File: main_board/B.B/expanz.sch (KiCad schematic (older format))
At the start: 22 parts, among them J1 Conn_01x04, J4 Conn_01x04, M1 Motor_DC, Q10 2N7002, Q7 SI3447CDV, U68 IRM-H936, U70 MH253ESO, U71 MH253ESO

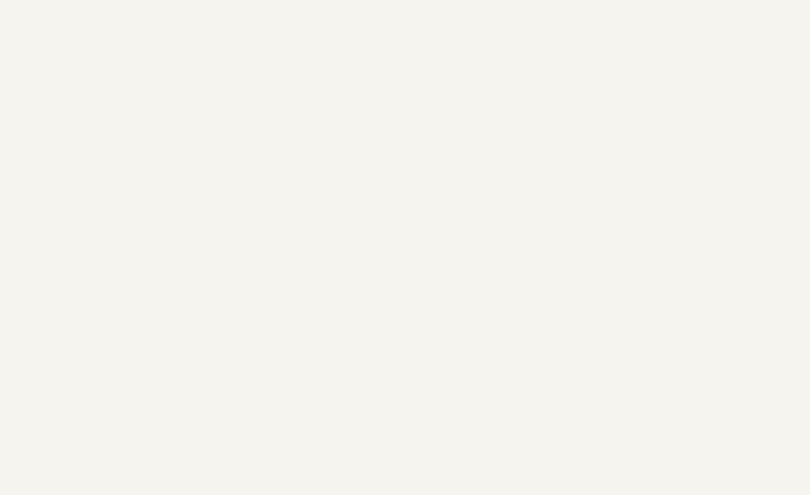
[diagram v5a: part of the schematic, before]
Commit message: opravy_a_dodatky_2
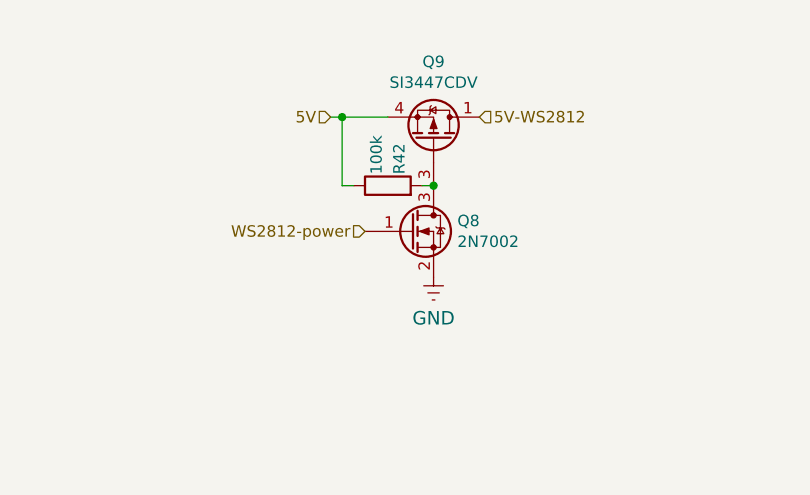
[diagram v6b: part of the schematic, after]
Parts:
- added Q8: 2N7002, Package_TO_SOT_SMD:SOT-23, symbol B.B-rescue:2N7002-Transistor_FET-B.B-rescue
- added Q9: SI3447CDV, BB:TSOP-6_1.5x3.0x0.95P, symbol B.B-rescue:Q_PMOS_DSG-B.B-rescue
- added R42: 100k, Resistor_SMD:R_0402_1005Metric, symbol B.B-rescue:R-Device-B.B-rescue
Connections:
- net 5V: now also Q9.4 (S), R42.1
- new net: Q8.3 (D), Q9.3 (G), R42.2
- new net 5V-WS2812: Q9.1 (D), Q9.2, Q9.5, Q9.6
- new net WS2812-power: Q8.1 (G)
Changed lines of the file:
@@
 EESchema Schematic File Version 4
-LIBS:B.B-cache
-EELAYER 29 0
+EELAYER 30 0
 EELAYER END
 $Descr A4 11693 8268
 encoding utf-8
-Sheet 7 8
+Sheet 8 8
 Title ""
 Date ""
@@
 $EndComp
 $Comp
+L B.B-rescue:GND-B.B-eagle-import #GND0137
+U 1 1 5F9DF814
+P 7750 3025
+AR Path="/5F9EE529/5F9DF814" Ref="#GND0137"  Part="1"
+AR Path="/5FA9DBB3/5F9DF814" Ref="#GND?"  Part="1"
+F 0 "#GND0137" H 7750 3025 50  0001 C CNN
+F 1 "GND" H 7750 2945 59  0000 C CNN
+F 2 "" H 7750 3025 50  0001 C CNN
+F 3 "" H 7750 3025 50  0001 C CNN
+	1    7750 3025
+	1    0    0    -1
+$EndComp
+Text HLabel 7950 2225 2    50   Input ~ 0
+5V-WS2812
+Text HLabel 7300 2225 0    50   Input ~ 0
+5V
+$Comp
+L B.B-rescue:R-Device-B.B-rescue R?
+U 1 1 5FAAB362
+P 7550 2525
+AR Path="/5F96CFDA/5FAAB362" Ref="R?"  Part="1"
+AR Path="/5F9EE529/5F9F24D4/5FAAB362" Ref="R?"  Part="1"
+AR Path="/5FA9DBB3/5F9F24D4/5FAAB362" Ref="R?"  Part="1"
+AR Path="/5F9EE529/5FAAB362" Ref="R42"  Part="1"
+F 0 "R42" H 7600 2475 50  0000 L CNN
+F 1 "100k" H 7600 2575 50  0000 L CNN
+F 2 "Resistor_SMD:R_0402_1005Metric" V 7480 2525 50  0001 C CNN
+F 3 "~" H 7550 2525 50  0001 C CNN
+F 4 "C25741" H 7550 2525 50  0001 C CNN "LCSC"
+	1    7550 2525
+	0    -1   -1   0
+$EndComp
+Wire Wire Line
+	7700 2525 7750 2525
+Wire Wire Line
+	7300 2225 7350 2225
+Wire Wire Line
+	7400 2525 7350 2525
+Wire Wire Line
+	7350 2525 7350 2225
+Connection ~ 7350 2225
+Wire Wire Line
+	7350 2225 7550 2225
+Text HLabel 7450 2725 0    50   Input ~ 0
+WS2812-power
+$Comp
 L B.B-rescue:MH253ESO-B.B-rescue U?
 U 1 1 5FB5B56F
@@
 $EndComp
 $Comp
+L B.B-rescue:Q_PMOS_DSG-B.B-rescue Q9
+U 1 1 602B1909
+P 7750 2325
+F 0 "Q9" V 8092 2325 50  0000 C CNN
+F 1 "SI3447CDV" V 8001 2325 50  0000 C CNN
+F 2 "BB:TSOP-6_1.5x3.0x0.95P" H 7950 2425 50  0001 C CNN
+F 3 "https://datasheet.lcsc.com/szlcsc/Vishay-Intertech-SI3447CDV-T1-E3_C145421.pdf" H 7750 2325 50  0001 C CNN
+F 4 "C144884" V 7750 2325 50  0001 C CNN "LCSC"
+	1    7750 2325
+	0    1    -1   0
+$EndComp
+$Comp
 L B.B-rescue:2N7002-Transistor_FET-B.B-rescue Q?
+U 1 1 5FBA8934
+P 7650 2725
+AR Path="/5F77B818/5FBA8934" Ref="Q?"  Part="1"
+AR Path="/5FA4C94D/5FBA8934" Ref="Q?"  Part="1"
+AR Path="/5F9EE529/5FBA8934" Ref="Q8"  Part="1"
+F 0 "Q8" H 7854 2771 50  0000 L CNN
+F 1 "2N7002" H 7854 2680 50  0000 L CNN
+F 2 "Package_TO_SOT_SMD:SOT-23" H 7850 2650 50  0001 L CIN
+F 3 "https://datasheet.lcsc.com/szlcsc/Changjiang-Electronics-Tech-CJ-CJ3134K_C110100.pdf" H 7650 2725 50  0001 L CNN
+F 4 "C8545" H 7650 2725 50  0001 C CNN "LCSC"
+F 5 "0;0;180" H 7650 2725 50  0001 C CNN "JLCPCB_CORRECTION"
+	1    7650 2725
+	1    0    0    -1
+$EndComp
+Connection ~ 7750 2525
+$Comp
+L B.B-rescue:2N7002-Transistor_FET-B.B-rescue Q?

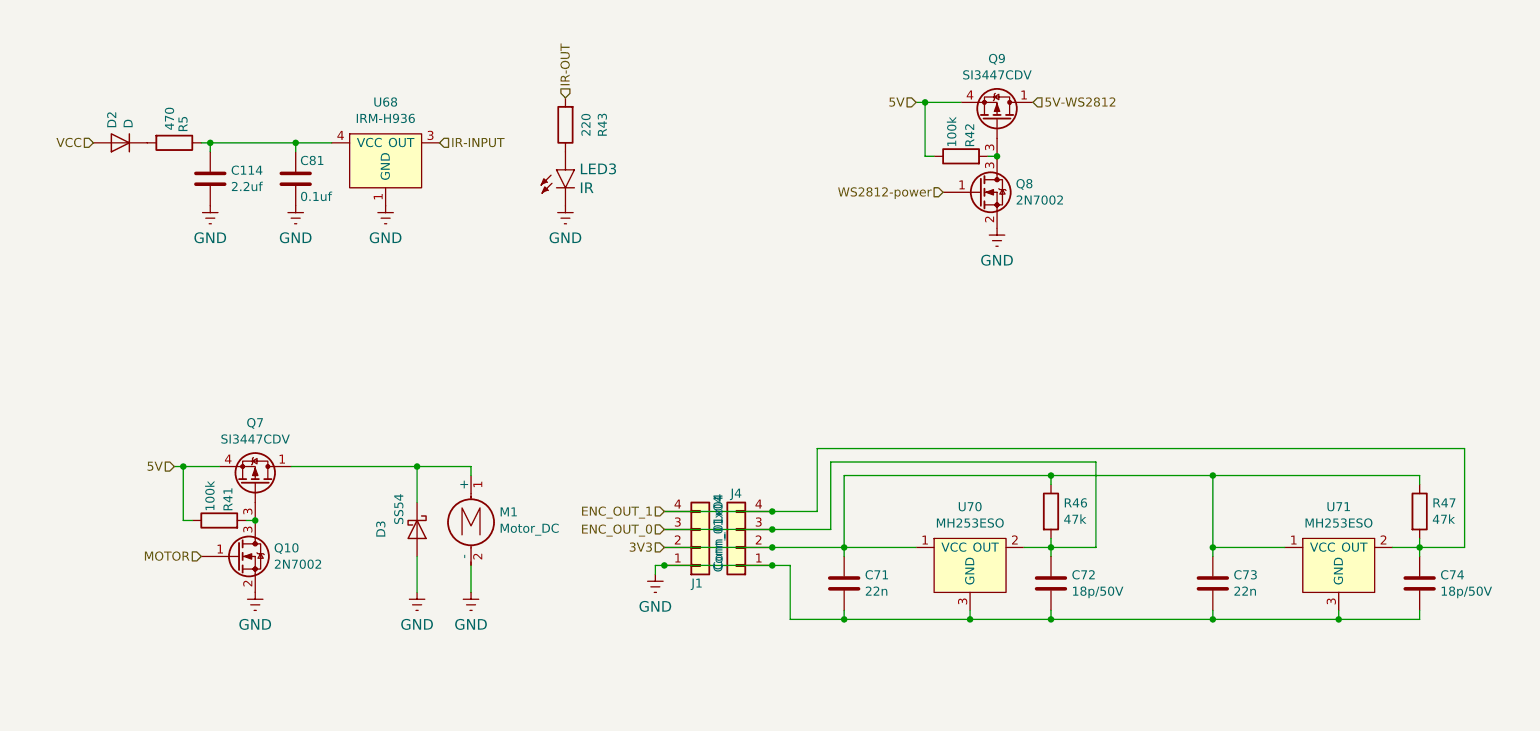
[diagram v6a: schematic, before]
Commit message: lucerna
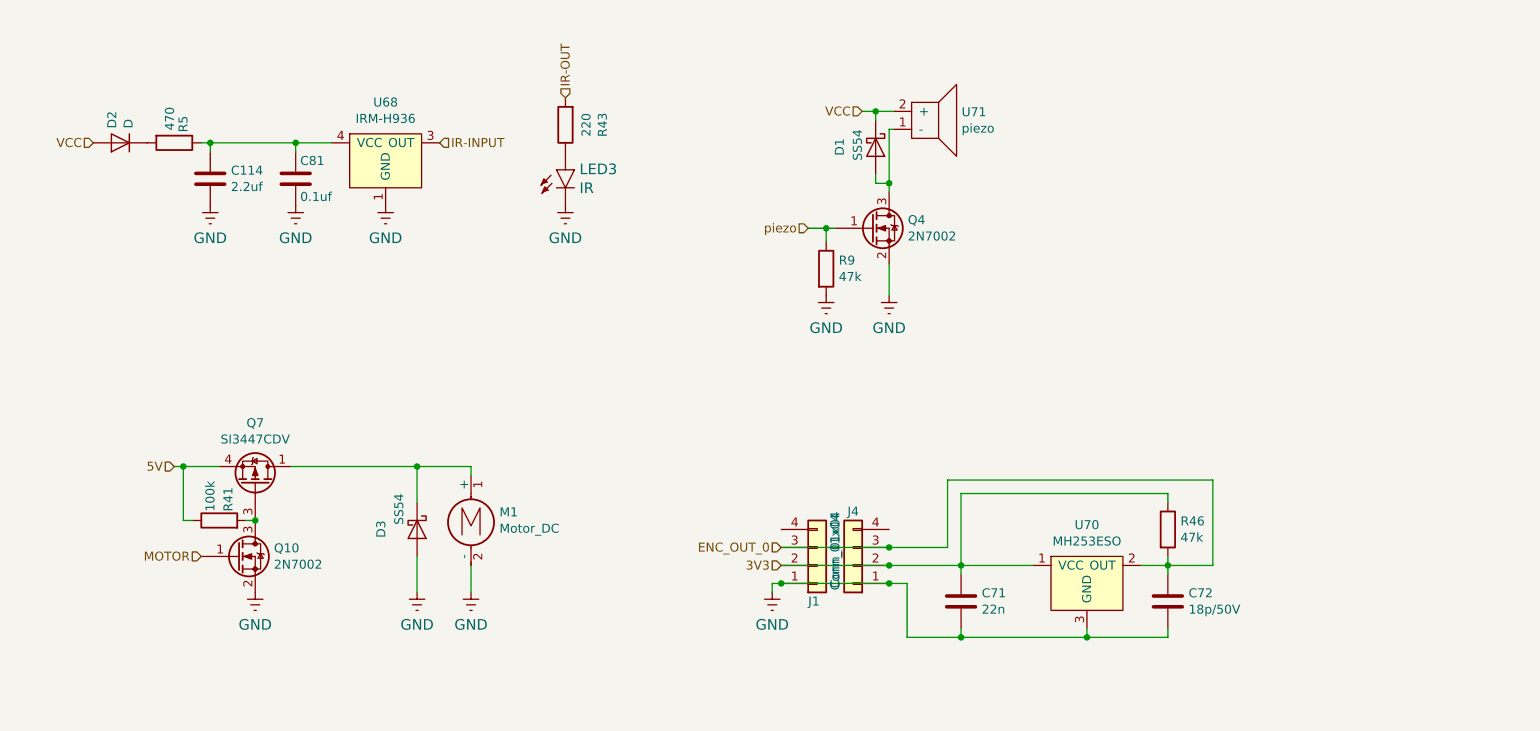
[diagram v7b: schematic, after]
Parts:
- removed C73: 22n, Capacitor_SMD:C_0402_1005Metric, symbol B.B-rescue:C-Device-B.B-rescue
- removed C74: 18p/50V, Capacitor_SMD:C_0402_1005Metric, symbol B.B-rescue:C-Device-B.B-rescue
- removed Q8: 2N7002, Package_TO_SOT_SMD:SOT-23, symbol B.B-rescue:2N7002-Transistor_FET-B.B-rescue
- removed Q9: SI3447CDV, BB:TSOP-6_1.5x3.0x0.95P, symbol B.B-rescue:Q_PMOS_DSG-B.B-rescue
- removed R42: 100k, Resistor_SMD:R_0402_1005Metric, symbol B.B-rescue:R-Device-B.B-rescue
- removed R47: 47k, Resistor_SMD:R_0402_1005Metric, symbol B.B-rescue:R-Device-B.B-rescue
- removed U71: MH253ESO, Package_TO_SOT_SMD:SOT-23, symbol B.B-rescue:MH253ESO-B.B-rescue
- added D1: SS54, BB:DO-214AC, symbol B.B-rescue:D_Schottky-Device-B.B-rescue
- added Q4: 2N7002, Package_TO_SOT_SMD:SOT-23, symbol B.B-rescue:2N7002-Transistor_FET-B.B-rescue
- added R9: 47k, Resistor_SMD:R_0402_1005Metric, symbol B.B-rescue:R-Device-B.B-rescue
- added U71: piezo, BB:piezo, symbol B.B-rescue:piezo
- M1: footprint Connector_PinHeader_1.00mm:PinHeader_1x02_P1.00mm_Vertical -> Connector_JST:JST_EH_B2B-EH-A_1x02_P2.50mm_Vertical
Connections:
- net VCC: now also D1.1 (K), U71.2 (+)
- net ENC_OUT_1: no longer names the net of J4.4 (Pin_4)
- net ENC_OUT_1: no longer J1.4 (Pin_4)
- new net: D1.2 (A), Q4.3 (D), U71.1 (-)
- new net piezo: Q4.1 (G), R9.1
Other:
- moved on the sheet: C71, C72, J1, J4, R46, U70

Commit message: presuny_konektoru
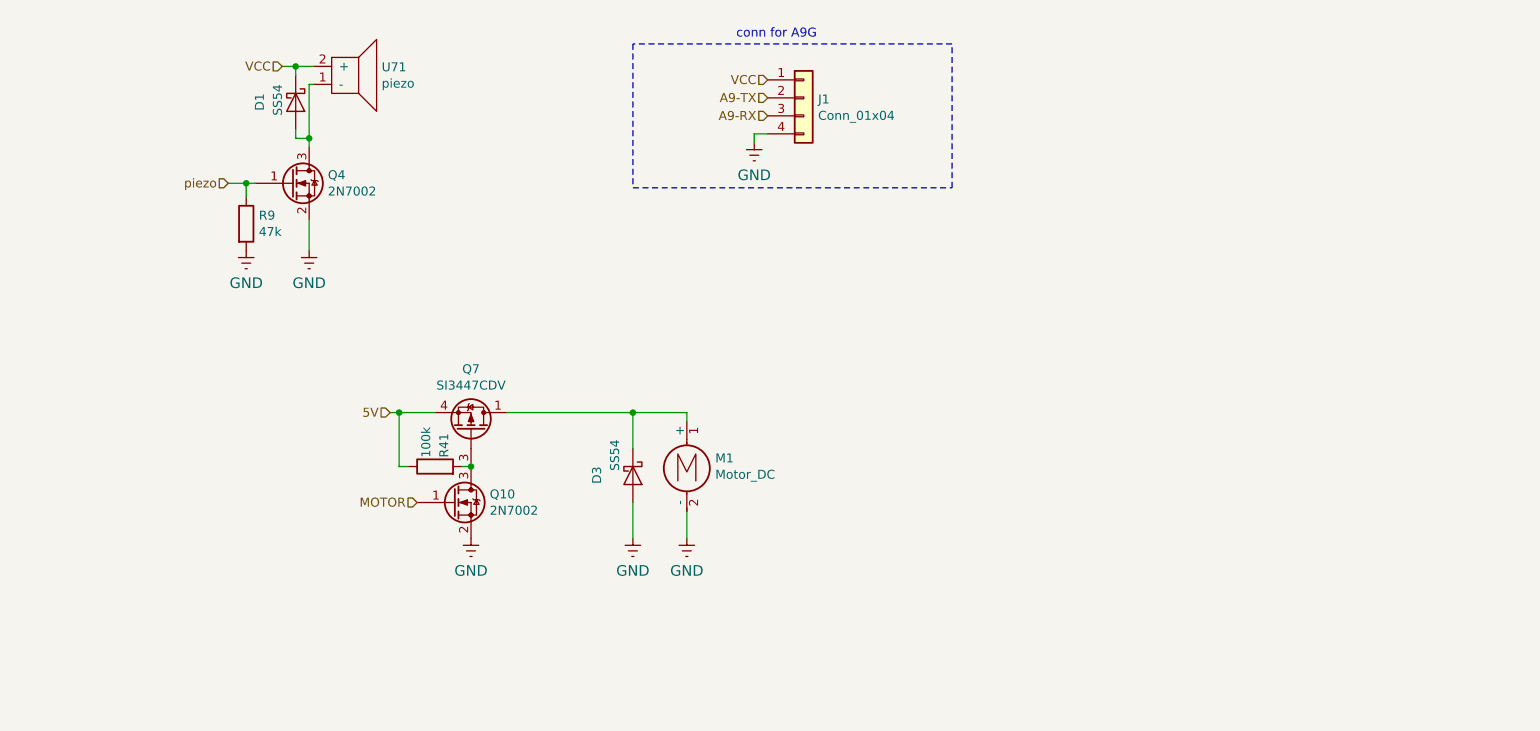
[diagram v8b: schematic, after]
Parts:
- removed C114: 2.2uf, Capacitor_SMD:C_0805_2012Metric, symbol B.B-rescue:C-Device-B.B-rescue
- removed C71: 22n, Capacitor_SMD:C_0402_1005Metric, symbol B.B-rescue:C-Device-B.B-rescue
- removed C72: 18p/50V, Capacitor_SMD:C_0402_1005Metric, symbol B.B-rescue:C-Device-B.B-rescue
- removed C81: 0.1uf, Resistor_SMD:R_0402_1005Metric, symbol B.B-rescue:C-Device-B.B-rescue
- removed D2: D, BB:SOD-323, symbol B.B-rescue:D-Device-B.B-rescue
- removed J1, J4: Conn_01x04, Connector_PinSocket_2.54mm:PinSocket_1x04_P2.54mm_Vertical, symbol B.B-rescue:Conn_01x04-Connector_Generic-B.B-rescue
- removed LED3: IR, LED_SMD:LED_0603_1608Metric, symbol B.B-rescue:LED-B.B-eagle-import
- removed R43: 220, Resistor_SMD:R_0402_1005Metric, symbol B.B-rescue:R-Device-B.B-rescue
- removed R46: 47k, Resistor_SMD:R_0402_1005Metric, symbol B.B-rescue:R-Device-B.B-rescue
- removed R5: 470, Resistor_SMD:R_0402_1005Metric, symbol B.B-rescue:R-Device-B.B-rescue
- removed U68: IRM-H936, BB:SMD-4_4.0x5.0x2.54P, symbol B.B-rescue:IRM-H936-B.B-rescue
- removed U70: MH253ESO, Package_TO_SOT_SMD:SOT-23, symbol B.B-rescue:MH253ESO-B.B-rescue
- added J1: Conn_01x04, Connector_PinHeader_2.54mm:PinHeader_1x04_P2.54mm_Vertical, symbol Connector_Generic:Conn_01x04
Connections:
- net VCC: now also J1.1 (Pin_1)
- new net A9-RX: J1.3 (Pin_3)
- new net A9-TX: J1.2 (Pin_2)
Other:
- note added: "conn for A9G"
- moved on the sheet: D1, D3, M1, Q10, Q4, Q7, R41, R9, U71
